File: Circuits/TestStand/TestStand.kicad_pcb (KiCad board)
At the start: 2 copper layers, 92.5 x 137.5 mm, 110 parts, among them IC1 STP85NF55, J1 Screw_Terminal_01x07, J10 Screw_Terminal_01x03, J11 Screw_Terminal_01x03, J12 Screw_Terminal_01x03, J13 Screw_Terminal_01x03, J14 Screw_Terminal_01x02, J15 Conn_Coaxial, J16 Screw_Terminal_01x02, J17 Screw_Terminal_01x02, J2 Screw_Terminal_01x07, J3 Screw_Terminal_01x07, J4 Screw_Terminal_01x03, J5 Screw_Terminal_01x03, J6 Screw_Terminal_01x03, J7 Screw_Terminal_01x03, J8 Screw_Terminal_01x03, J9 Screw_Terminal_01x03, Q1 MMBT4403-7-F, Q2 MMBT4403-7-F, Q3 MMBT4403-7-F, U1 HX711, U2 HX711, U3 HX711, U4 Teensy4.1, U5 LP2980IM5X-3.3/NOPB, U6 MAX31855KASA, U7 NRF24L01, U8 LP2980IM5X-3.3/NOPB, Y1 16Mhz

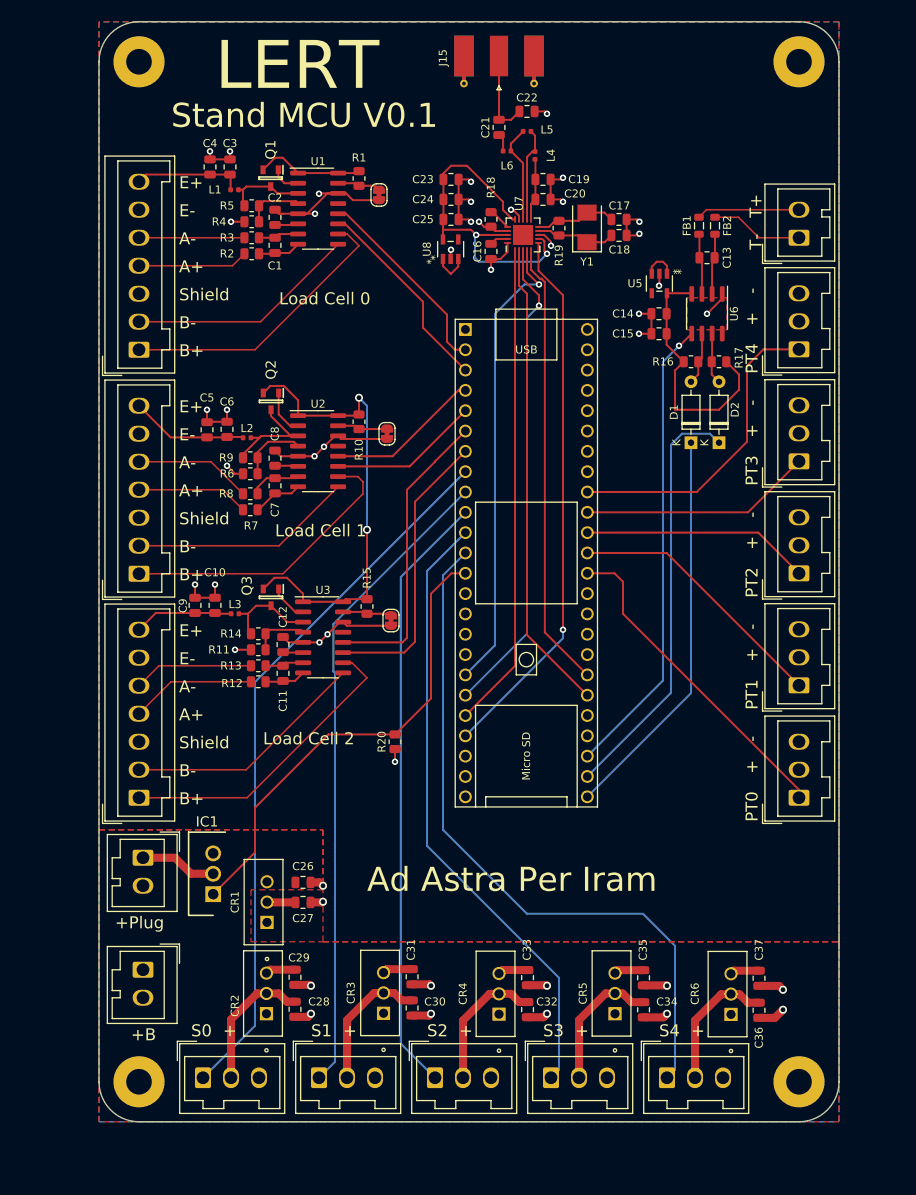
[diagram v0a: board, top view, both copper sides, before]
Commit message: switched to the true connectors, did some rearranging, largely backwards progress :)
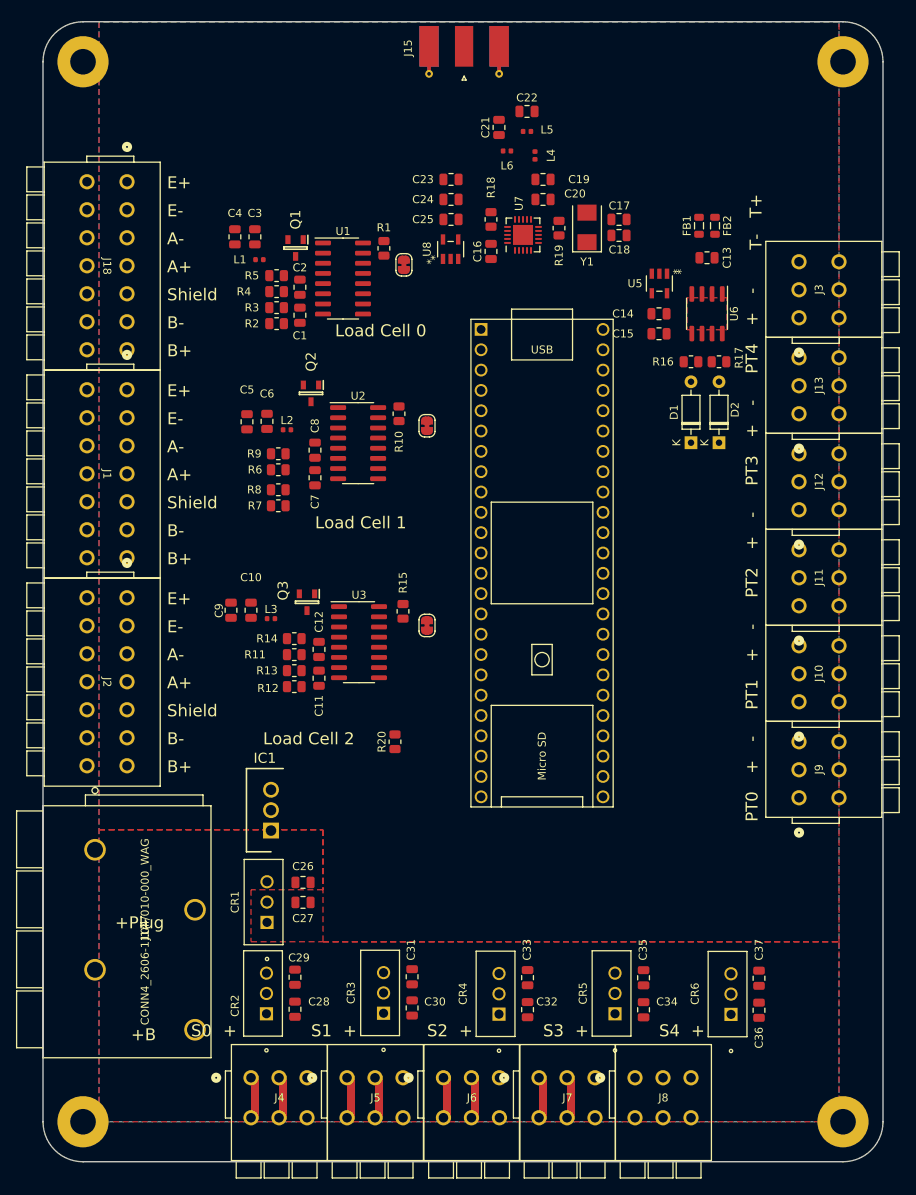
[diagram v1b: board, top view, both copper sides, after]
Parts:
- removed J16, J17: Screw_Terminal_01x02, Connector_Wago:Wago_734-132_1x02_P3.50mm_Vertical
- added J18: 2601-1107, Library:CONN7_2601-1107_WAG, F.Cu at (26.0, 83.0)
- J1, J2: value Screw_Terminal_01x07 -> 2601-1107; footprint Connector_Wago:Wago_734-137_1x07_P3.50mm_Vertical -> Library:CONN7_2601-1107_WAG
- J10, J11, J12, J13, J4, J5, J6, J7, J8, J9: footprint Connector_Wago:Wago_734-133_1x03_P3.50mm_Vertical -> Library:CONN3_2601-1103_WAG
- J14: value Screw_Terminal_01x02 -> CONN4_2606-1104/010-000_WAG; footprint Connector_Wago:Wago_734-132_1x02_P3.50mm_Vertical -> Library:2606-1104&slash_010-000
- J3: value Screw_Terminal_01x07 -> Screw_Terminal_01x03; footprint Connector_Wago:Wago_734-137_1x07_P3.50mm_Vertical -> Library:CONN3_2601-1103_WAG
- moved J14 116.6 mm to (22.0, 166.5), turned to -90 degrees
- moved J3 102.0 mm to (110.0, 100.0)
- moved IC1 10.7 mm to (44.0, 164.1)
- moved R2 9.27 mm to (44.7, 100.7)
- moved R3 9.27 mm to (44.7, 98.7)
- moved R4 9.27 mm to (44.7, 96.7)
- moved R5 9.27 mm to (44.7, 94.7)
- moved C1 9.27 mm to (47.6, 99.7)
- moved C2 9.27 mm to (47.6, 96.2)
- moved C3 9.27 mm to (42.0, 89.9)
- moved C4 9.27 mm to (39.5, 89.9)
- moved JP1 9.27 mm to (60.6, 93.4)
- moved L1 9.27 mm to (42.5, 92.7)
- moved Q1 9.27 mm to (47.1, 91.3)
- moved R1 9.27 mm to (58.1, 91.3)
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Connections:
- FB1 pad 1: /T+ -> Net-(J3-1_1)
- IC1 pad 2: Net-(IC1-D) -> /DRAIN
- J1 pad 1: /B+ -> /E1+
- J1 pad 2: /B- -> /E1+
- J1 pad 4: /A+ -> GND
- J1 pad 5: /A- -> /A1-
- J1 pad 6: GND -> /A1-
- J1 pad 7: /E+ -> /A1+
- J10 pad 2: +5V -> /PT1
- J10 pad 3: GND -> +5V
- J11 pad 2: +5V -> /PT2
- J11 pad 3: GND -> +5V
- J12 pad 2: +5V -> /PT3
- J12 pad 3: GND -> +5V
- J13 pad 2: +5V -> /PT4
- J13 pad 3: GND -> +5V
- J14 pad 1: /T- -> +BATT
- J14 pad 2: /T+ -> GND
- J2 pad 1: /B1+ -> /E2+
- J2 pad 2: /B1- -> /E2+
- J2 pad 4: /A1+ -> GND
- J2 pad 5: /A1- -> /A2-
- J2 pad 6: GND -> /A2-
- J2 pad 7: /E1+ -> /A2+
- J3 pad 1: /B2+ -> Net-(J3-1_1)
- J3 pad 2: /B2- -> Net-(J3-1_1)
- J3 pad 3: GND -> /T-
- J3 pad 4: /A2+ -> /T-
- J3 pad 5: /A2- -> unconnected-(J3-3_1-Pad5)
- J3 pad 6: GND -> unconnected-(J3-3_2-Pad6)
- J4 pad 2: /+S0 -> /PWM0
- J4 pad 3: GND -> /+S0
- J5 pad 2: /+S1 -> /PWM1
- J5 pad 3: GND -> /+S1
- J6 pad 2: /+S2 -> /PWM2
- J6 pad 3: GND -> /+S2
- J7 pad 2: /+S3 -> /PWM3
- J7 pad 3: GND -> /+S3
- J8 pad 2: /+S4 -> /PWM4
- J8 pad 3: GND -> /+S4
- J9 pad 2: +5V -> /PT0
- J9 pad 3: GND -> +5V
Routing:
- net GND: track 150.9 -> 0.00 mm, vias 45 -> 0
- net /PWM4: track 87.7 -> 0.00 mm
- net /PWM0: track 89.3 -> 5.00 mm
- net +5V: track 84.1 -> 0.00 mm, vias 2 -> 0
- net /PWM1: track 81.0 -> 5.00 mm
- net /PWM3: track 77.4 -> 5.00 mm
- net /PWM2: track 75.9 -> 5.00 mm
- net /rIRQ: track 67.9 -> 0.00 mm, vias 1 -> 0
- net /rCE: track 60.7 -> 0.00 mm
- net /rSCK: track 60.2 -> 0.00 mm, vias 1 -> 0
- net /rCSN: track 59.1 -> 0.00 mm
- net /GP: track 59.1 -> 0.00 mm
- net /rMOSI: track 58.6 -> 0.00 mm, vias 1 -> 0
- net /tcSCK: track 58.3 -> 0.00 mm, vias 1 -> 0
- net /rMISO: track 56.1 -> 0.00 mm
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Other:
- board size 92.5 x 137.5 mm -> 105 x 142.5 mm
- board text removed: ":3"
- board text removed: "Ad Astra Per Iram"
- board text removed: "LERT"
- board text removed: "Stand MCU V0.1"
